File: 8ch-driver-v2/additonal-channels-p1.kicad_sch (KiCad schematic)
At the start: 42 parts, among them Q3 2N7002E, Q4 2N7002E, Q5 2N7002E, U3 DRV104PWP, U4 DRV104PWP, U5 DRV104PWP

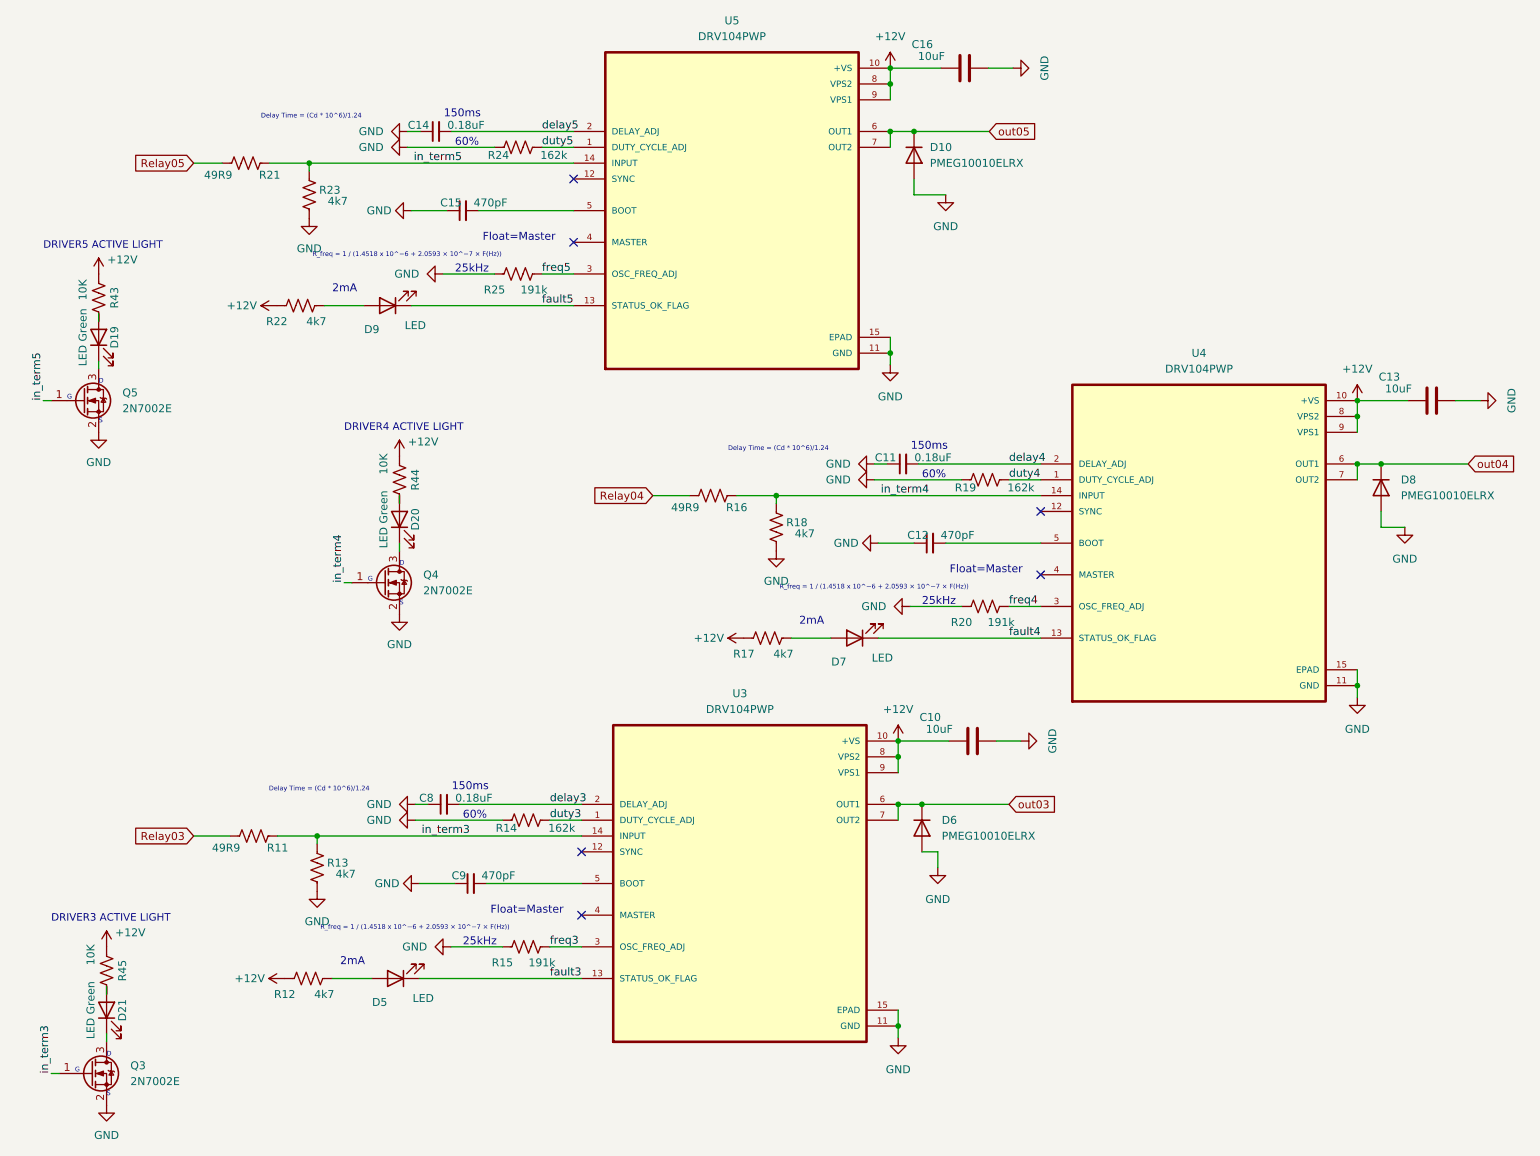
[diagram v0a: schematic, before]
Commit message: mucho mas progresso
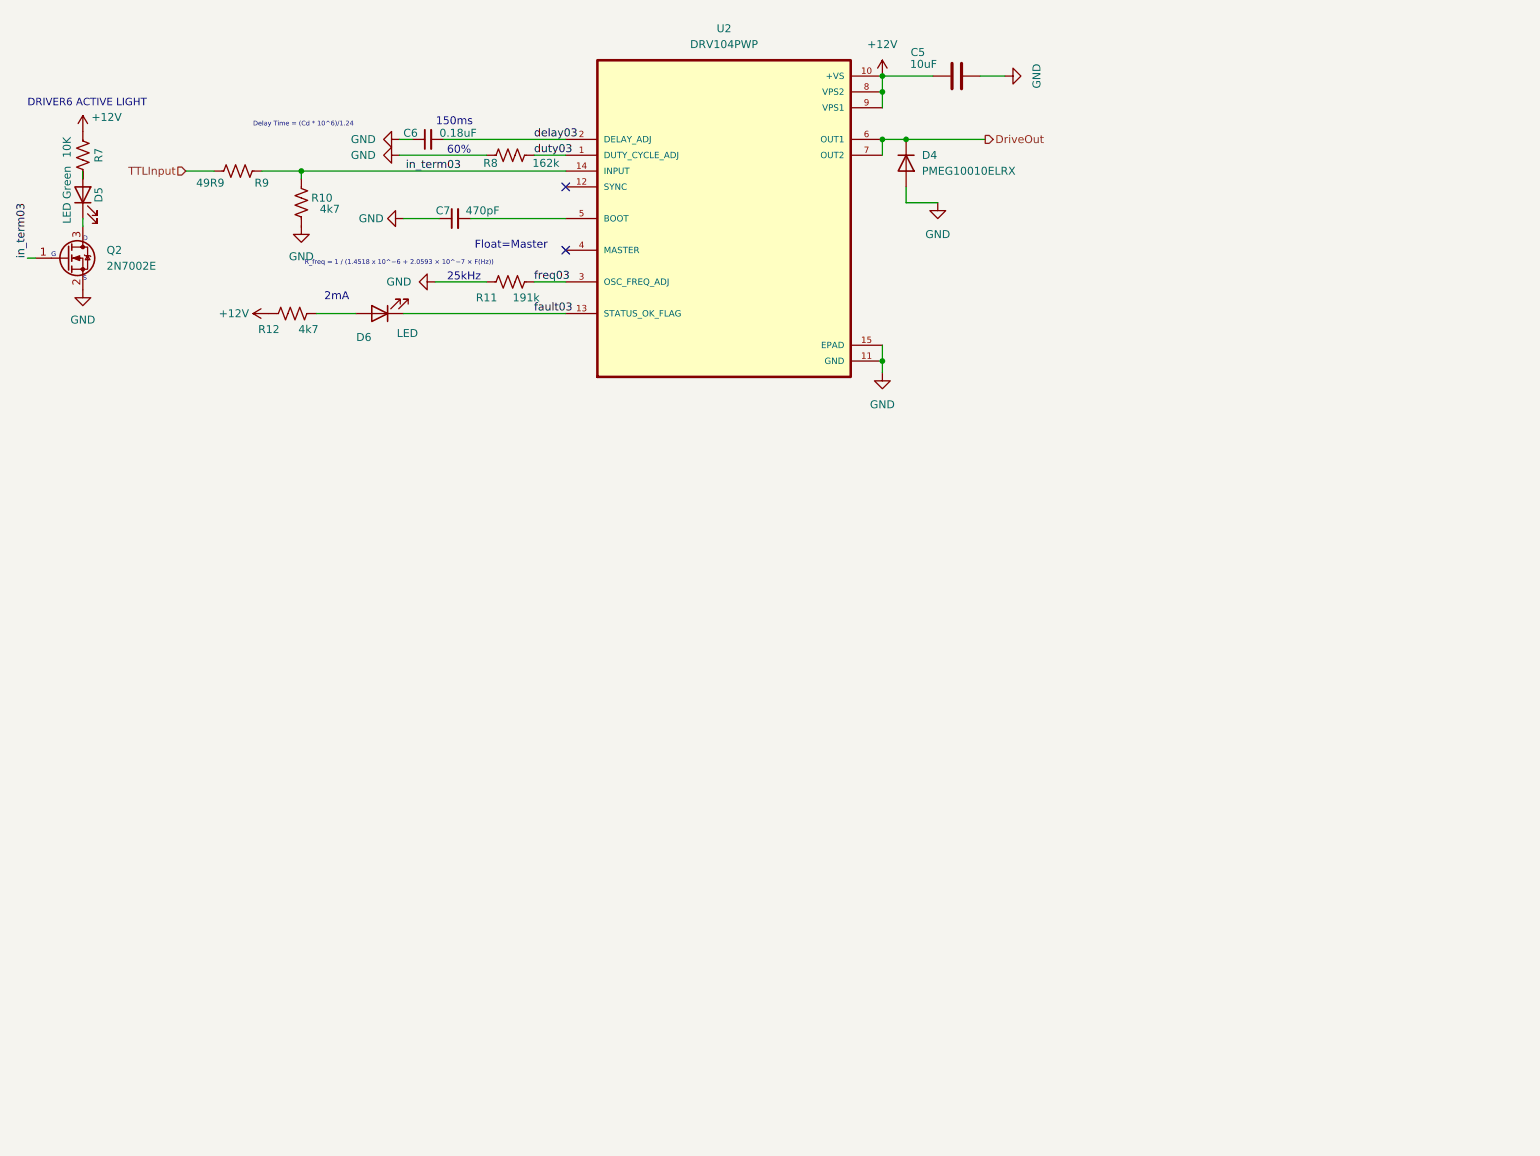
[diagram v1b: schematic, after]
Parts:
- removed C10, C13, C16: 10uF, Capacitor_SMD:C_1210_3225Metric, symbol Device:C
- removed C11, C14, C8: 0.18uF, Capacitor_SMD:C_1206_3216Metric, symbol Device:C_Small
- removed C12, C15, C9: 470pF, Capacitor_SMD:C_1206_3216Metric, symbol Device:C_Small
- removed D10, D6, D8: PMEG10010ELRX, Diode_SMD:Nexperia_CFP3_SOD-123W, symbol Device:D
- removed D19, D20, D21: LED Green, LED_SMD:LED_0805_2012Metric, symbol Device:LED
- removed D7, D9: LED, LED_SMD:LED_0805_2012Metric, symbol Device:LED
- removed Q3, Q4, Q5: 2N7002E, Package_TO_SOT_SMD:SOT-23, symbol Transistor_FET:2N7002E
- removed R13, R17, R18, R22, R23: 4k7, Resistor_SMD:R_1206_3216Metric, symbol Device:R_US
- removed R14, R19, R24: 162k, Resistor_SMD:R_1206_3216Metric, symbol Device:R_US
- removed R15, R20, R25: 191k, Resistor_SMD:R_1206_3216Metric, symbol Device:R_US
- removed R16, R21: 49R9, Resistor_SMD:R_1206_3216Metric, symbol Device:R_US
- removed R43, R44, R45: 10K, Resistor_SMD:R_1206_3216Metric, symbol Device:R_US
- removed U3, U4, U5: DRV104PWP, Solenoid_Driver:IC_TPS27S100BPWPR, symbol DRV104PWP:DRV104PWP
- added C5: 10uF, Capacitor_SMD:C_1210_3225Metric, symbol Device:C
- added C6: 0.18uF, Capacitor_SMD:C_1206_3216Metric, symbol Device:C_Small
- added C7: 470pF, Capacitor_SMD:C_1206_3216Metric, symbol Device:C_Small
- added D4: PMEG10010ELRX, Diode_SMD:Nexperia_CFP3_SOD-123W, symbol Device:D
- added D6: LED, LED_SMD:LED_0805_2012Metric, symbol Device:LED
- added Q2: 2N7002E, Package_TO_SOT_SMD:SOT-23, symbol Transistor_FET:2N7002E
- added R10: 4k7, Resistor_SMD:R_1206_3216Metric, symbol Device:R_US
- added R7: 10K, Resistor_SMD:R_1206_3216Metric, symbol Device:R_US
- added R8: 162k, Resistor_SMD:R_1206_3216Metric, symbol Device:R_US
- added R9: 49R9, Resistor_SMD:R_1206_3216Metric, symbol Device:R_US
- added U2: DRV104PWP, Solenoid_Driver:IC_TPS27S100BPWPR, symbol DRV104PWP:DRV104PWP
- D5: value LED -> LED Green
- R11: value 49R9 -> 191k; PartNum RC0805FR-0749R9L -> RC0805FR-07191KL
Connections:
- net Relay03 is gone; now on net GND: R11.1
- net +12V: now also C5.1, R7.1, U2.10 (+VS), U2.8 (VPS2), U2.9 (VPS1)
- net GND: now also C5.2, C6.1, C7.1, D4.2 (A), Q2.2 (S), R10.1, R8.1, U2.11 (GND), U2.15 (EPAD)
- net at D5.2 (A): now also R7.2; no longer R12.2
- net fault3: no longer names the net of D5.1 (K)
- net fault3: now also Q2.3 (D)
- net in_term3 renamed freq03
- net freq03: now also U2.3 (OSC_FREQ_ADJ)
- new net: C7.2, U2.5 (BOOT)
- new net: D6.2 (A), R12.2
- new net DriveOut: D4.1 (K), U2.6 (OUT1), U2.7 (OUT2)
- new net TTLInput: R9.1
- new net delay03: C6.2, U2.2 (DELAY_ADJ)
- new net duty03: R8.2, U2.1 (DUTY_CYCLE_ADJ)
- new net fault03: D6.1 (K), U2.13 (STATUS_OK_FLAG)
- new net in_term03: Q2.1 (G), R10.2, R9.2, U2.14 (INPUT)
- no-connect marks 6 -> 2
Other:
- note added: "DRIVER6 ACTIVE LIGHT"
- note removed: "DRIVER3 ACTIVE LIGHT"
- note removed: "DRIVER4 ACTIVE LIGHT"
- note removed: "DRIVER5 ACTIVE LIGHT"
